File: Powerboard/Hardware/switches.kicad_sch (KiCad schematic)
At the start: 15 parts, among them J4 Conn_01x02_Male, J5 RBUS, J6 Conn_01x02_Male, Q1 RSJ250P10TL, Q2 RSJ250P10TL, Q3 RSJ250P10TL, Q4 RSJ250P10TL, U6 LTC4412xS6, U7 LTC4412xS6

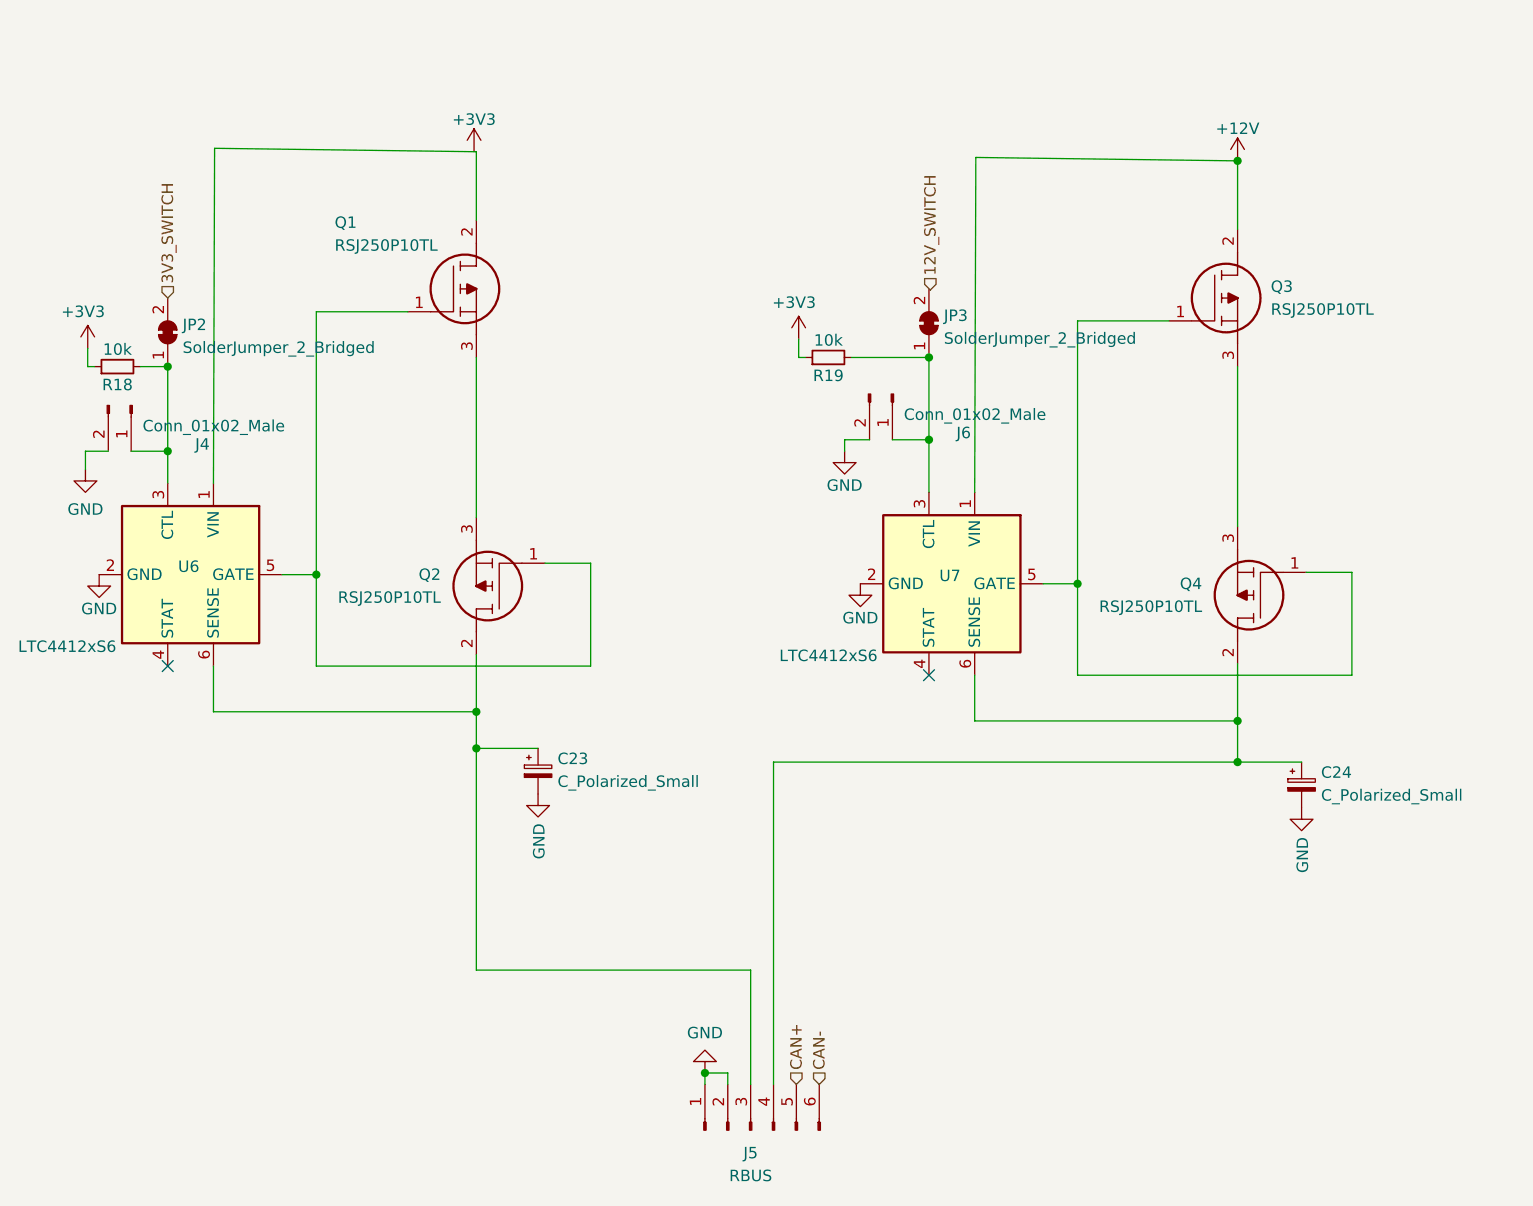
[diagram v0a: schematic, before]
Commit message: latest
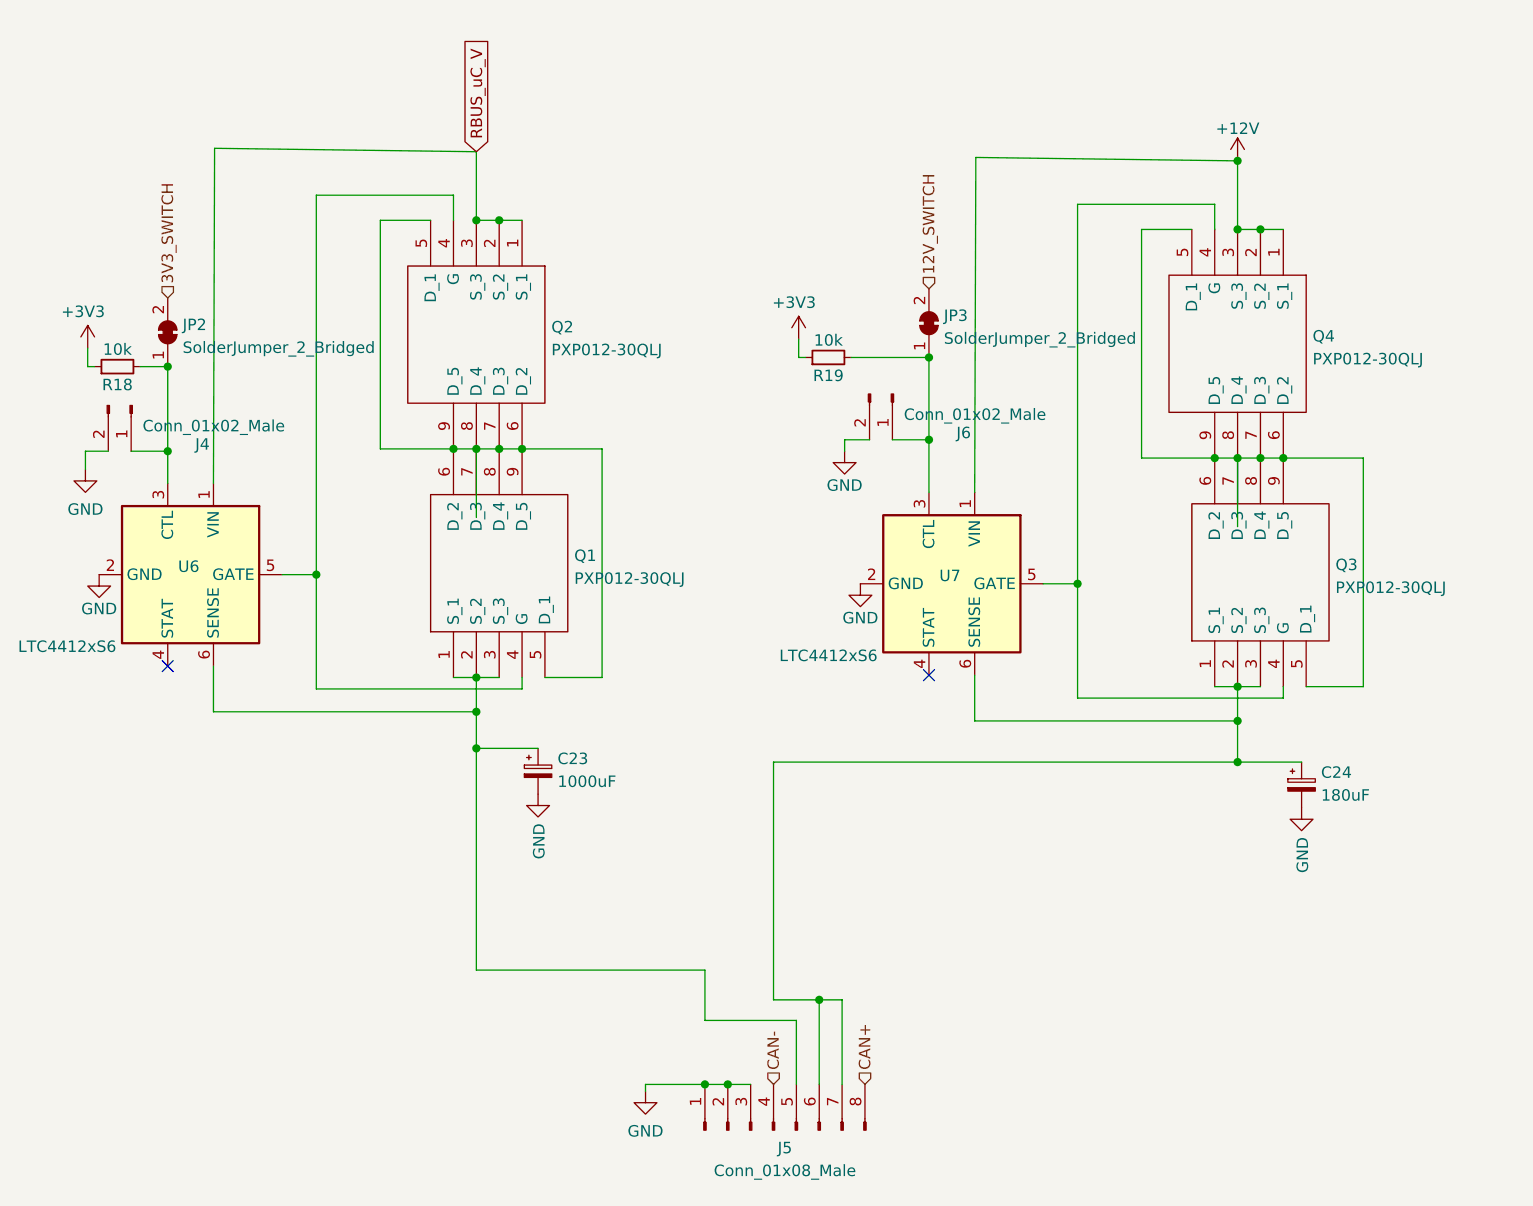
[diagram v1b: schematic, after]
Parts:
- removed J5: RBUS, Connector_Molex:Molex_Mini-Fit_Jr_5566-06A_2x03_P4.20mm_Vertical, symbol Connector:Conn_01x06_Male
- removed Q1, Q2, Q3, Q4: RSJ250P10TL, Package_TO_SOT_SMD:TO-263-3_TabPin2, symbol iclr:RSJ250P10TL
- added J5: Conn_01x08_Male, Connector_Molex:Molex_Mini-Fit_Jr_5569-08A2_2x04_P4.20mm_Horizontal, symbol Connector:Conn_01x08_Male
- added Q1, Q2, Q3, Q4: PXP012-30QLJ, iclr:PXP01230QLJ, symbol iclr:PXP012-30QLJ
- C23: value C_Polarized_Small -> 1000uF
- C24: value C_Polarized_Small -> 180uF
- J4, J6: footprint Connector_PinHeader_2.54mm:PinHeader_1x02_P2.54mm_Vertical -> Connector_Molex:Molex_Nano-Fit_105313-xx02_1x02_P2.50mm_Horizontal
- JP2, JP3: footprint Jumper:SolderJumper-3_P1.3mm_Bridged2Bar12_RoundedPad1.0x1.5mm -> Jumper:SolderJumper-2_P1.3mm_Bridged_RoundedPad1.0x1.5mm
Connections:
- net +12V: now also Q4.1 (S_1), Q4.2 (S_2), Q4.3 (S_3)
- net 12V_SWITCH: now also JP3.2 (B)
- net CAN+: now also J5.8 (Pin_8)
- net CAN-: now also J5.4 (Pin_4)
- net GND: now also J5.1 (Pin_1), J5.2 (Pin_2), J5.3 (Pin_3)
- net RBUS_uC_V: now reaches U6.1 (VIN)
- net RBUS_uC_V: now also Q2.1 (S_1), Q2.2 (S_2), Q2.3 (S_3)
- net at U6.5 (GATE): now also Q1.4 (G), Q2.4 (G)
- net at C23.1, U6.6 (SENSE): now also J5.5 (Pin_5), Q1.1 (S_1), Q1.2 (S_2), Q1.3 (S_3)
- net at C24.1, U7.6 (SENSE): now also J5.6 (Pin_6), J5.7 (Pin_7), Q3.1 (S_1), Q3.2 (S_2), Q3.3 (S_3)
- net at U7.5 (GATE): now also Q3.4 (G), Q4.4 (G)
- new net: Q3.5 (D_1), Q3.6 (D_2), Q3.7 (D_3), Q3.8 (D_4), Q3.9 (D_5), Q4.5 (D_1), Q4.6 (D_2), Q4.7 (D_3), Q4.8 (D_4), Q4.9 (D_5)
- new net: Q1.5 (D_1), Q1.6 (D_2), Q1.7 (D_3), Q1.8 (D_4), Q1.9 (D_5), Q2.5 (D_1), Q2.6 (D_2), Q2.7 (D_3), Q2.8 (D_4), Q2.9 (D_5)
